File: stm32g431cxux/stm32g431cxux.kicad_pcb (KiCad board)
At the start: 2 copper layers, 17.8 x 31.8 mm, 22 parts, among them J1 USB2.0_C_v3, J2 ProMicro-LeftPin-NoGND, J3 ProMicro-RightPin, SW1 SW_Push, U1 AMS1117-3.3, U2 STM32G431CBUx

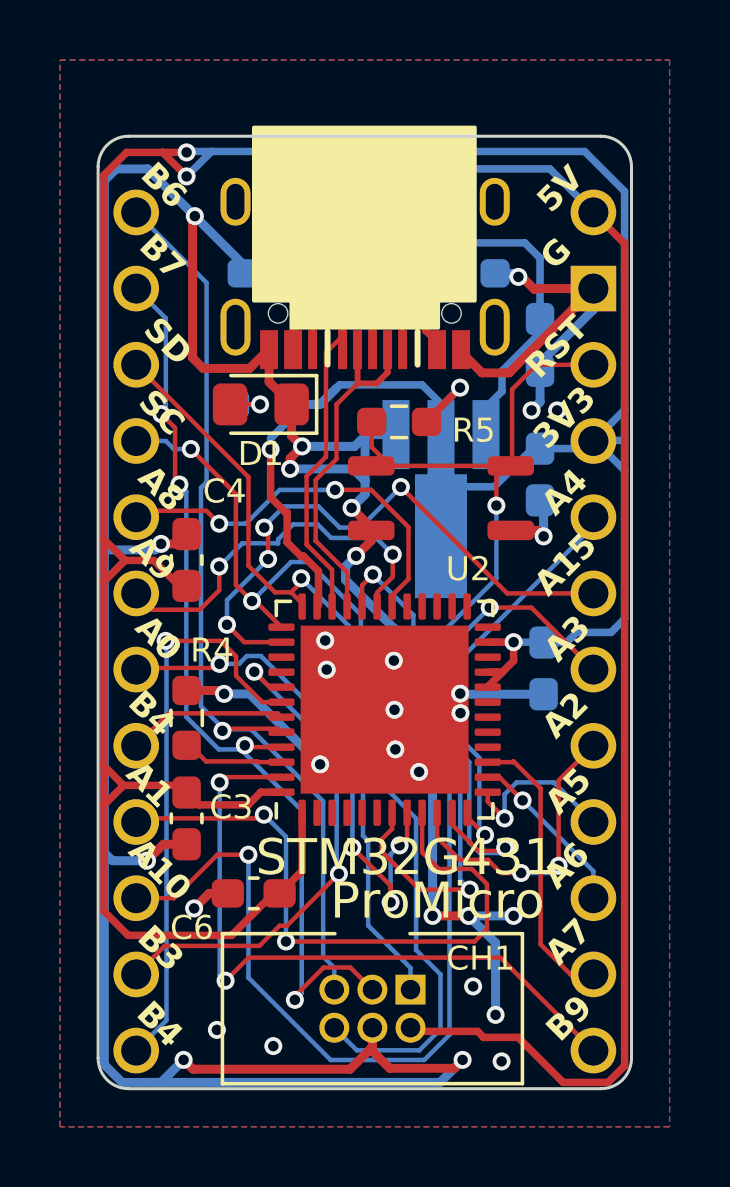
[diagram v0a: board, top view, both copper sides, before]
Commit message: stm32g03xfxp/v1.3.0
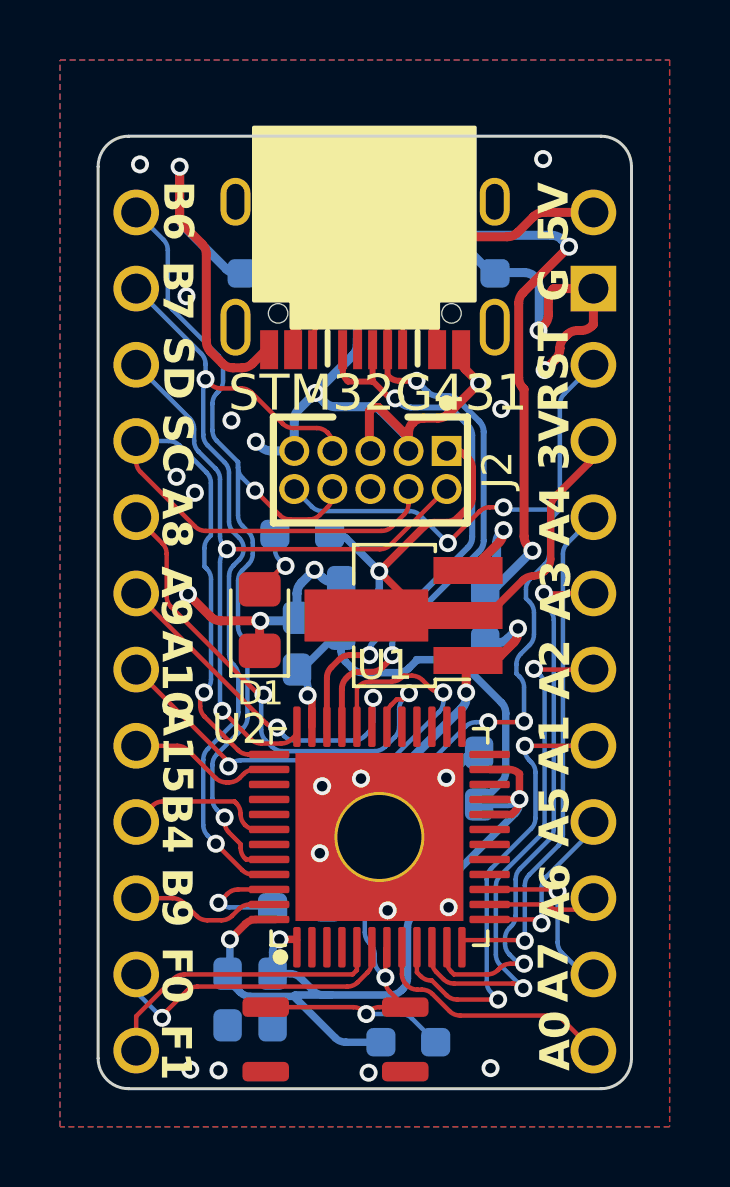
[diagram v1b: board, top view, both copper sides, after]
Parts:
- removed CH1: DAPLink-SWD-Recv-6Pin, $74th:BoxPinHeader_2x03_P1.27mm_Vertical
- added J2: SWD-MCU_Side-10Pin, $74th:SWD_2x05_P1.27mm, F.Cu at (68.8, 46.1)
- C3: renamed from C6; moved to B.Cu
- C5: renamed from C4; moved to B.Cu
- C6: renamed from C3; moved to B.Cu
- R4, R5: moved to B.Cu
- U1: footprint $74th:Regulator_AMS1117_SOT-89 -> Package_TO_SOT_SMD:SOT-89-3_Handsoldering; moved to F.Cu
- U2: footprint Package_DFN_QFN:QFN-48-1EP_7x7mm_P0.5mm_EP5.6x5.6mm -> $74th:QFN-48-1EP_7x7mm_P0.5mm_EP5.6x5.6mm
- moved R5 20.7 mm to (67.5, 65.8), turned to 0 degrees
- moved SW1 18.4 mm to (65.1, 65.7)
- moved C5 14.5 mm to (61.5, 64.2), turned to -90 degrees
- moved G*** 13.5 mm to (70.4, 60.9)
- moved C2 9.25 mm to (70.1, 51.5)
- moved C3 8.33 mm to (63.8, 52.6), turned to 90 degrees
- moved C1 8.10 mm to (65.3, 51.4), turned to 90 degrees
- moved R4 7.36 mm to (63.9, 61.3), turned to 0 degrees
- moved D1 7.19 mm to (62.5, 51.7), turned to 90 degrees
- moved C6 6.68 mm to (63.0, 64.2)
- moved R3 4.52 mm to (64.0, 48.8)
- moved C4 4.43 mm to (69.8, 57.1), turned to 90 degrees
- moved U2 4.25 mm to (66.5, 58.9)
- moved U1 4.18 mm to (67.0, 51.5), turned to 180 degrees
- moved REF** 0.20 mm to (59.9, 40.6)
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- renumbered C2 to C1, C1 to C2, C5 to C4, J2 to J3, J3 to J4, R2 to R1, R1 to R2
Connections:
- U2 pad 10: /18/A0 -> /19/A1
- U2 pad 11: /19/A1 -> /20/A2
- U2 pad 32: /7 -> /4/A6
- U2 pad 38: /20/A2 -> /5
- U2 pad 41: /8/A9 -> unconnected-(U2-PB3-Pad41)
- U2 pad 42: /9/A9 -> /6/A7
- U2 pad 43: /5 -> unconnected-(U2-PB5-Pad43)
- U2 pad 47: /10/A10 -> /7
- U2 pad 5: unconnected-(U2-PF0-Pad5) -> /9/A9
- U2 pad 6: unconnected-(U2-PF1-Pad6) -> /8/A9
- U2 pad 8: /4/A6 -> /10/A10
- U2 pad 9: /6/A7 -> /18/A0
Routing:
- net GND: track 139.0 -> 87.5 mm, vias 32 -> 30
- net +3V3: track 116.7 -> 68.4 mm
- net +5V: track 56.0 -> 20.9 mm
- net /7: track 34.2 -> 4.86 mm, vias 2 -> 0
- net /6/A7: track 21.2 -> 5.26 mm, vias 2 -> 0
- net /NRST: track 32.8 -> 46.9 mm, vias 2 -> 6
- net /10/A10: track 22.7 -> 9.04 mm, vias 2 -> 0
- net /9/A9: track 19.2 -> 9.88 mm, vias 1 -> 0
- net /D-: track 11.5 -> 20.0 mm, vias 0 -> 2
- net Net-(U1-VI): track 14.6 -> 23.1 mm, vias 0 -> 3
- net /SWCLK: track 33.1 -> 25.6 mm, vias 2 -> 1
- net /8/A9: track 17.2 -> 10.1 mm, vias 2 -> 1
- net /D+: track 12.9 -> 19.5 mm, vias 0 -> 2
- net /18/A0: track 9.95 -> 15.7 mm
- net /2/I2C_SDA: track 13.2 -> 17.0 mm
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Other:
- board text added: "3V"
- board text added: "F0"
- board text added: "F1"
- board text added: "v1.1.0"
- board text removed: "3V3"
- board text removed: "B3"
- board text removed: "v1.0.0"
